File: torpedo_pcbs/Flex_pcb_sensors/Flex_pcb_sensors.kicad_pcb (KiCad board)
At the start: 2 copper layers, 38.1 x 23.8 mm, 10 parts, among them IC1 VL53L1CXV0FY_1, J1 Conn_01x04, J2 Conn_01x04, J3 mounting, U1 MS583702BA01-50

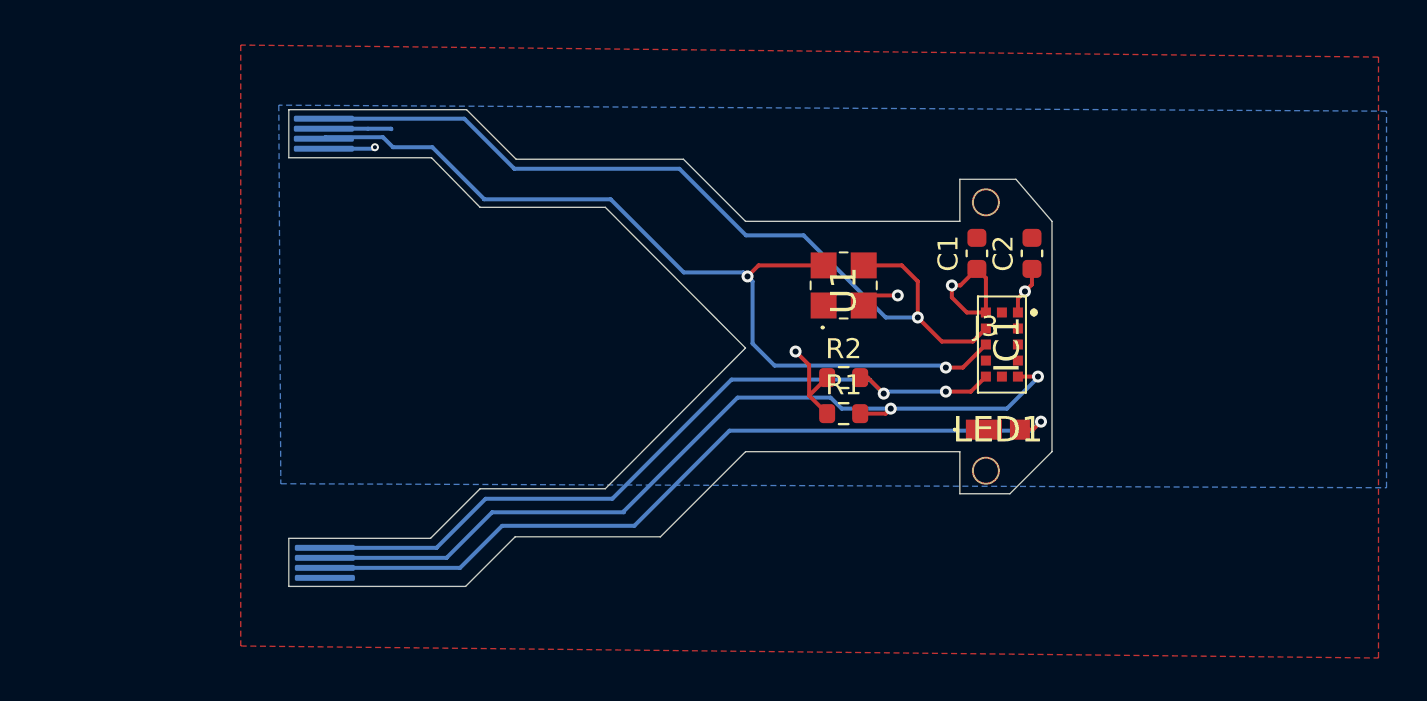
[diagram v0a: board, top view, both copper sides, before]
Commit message: everything is connected
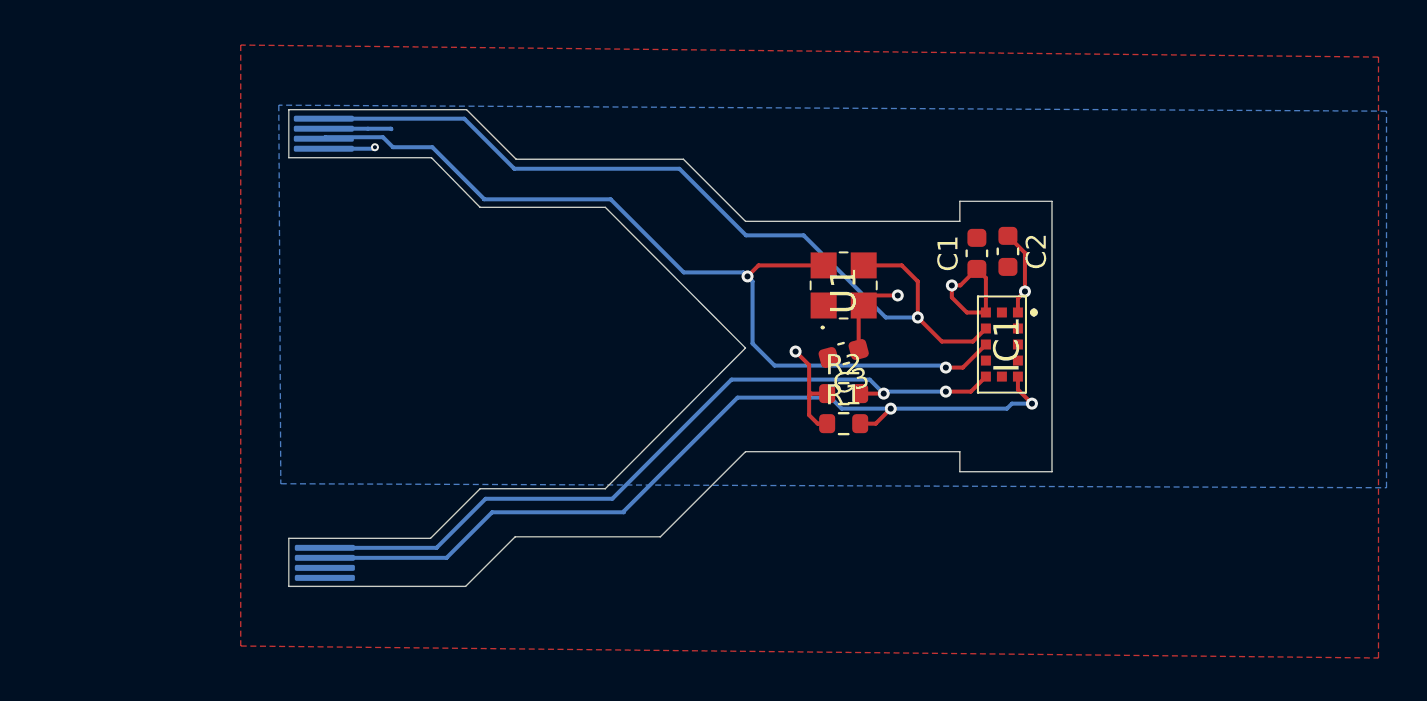
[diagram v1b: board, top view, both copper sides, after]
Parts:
- removed J3: mounting, MountingEquipment:small mounting holes
- removed LED1: 158301260A, SamacSys_Parts:158301260A
- added C3: 100nf, Capacitor_SMD:C_0603_1608Metric, F.Cu at (164.7, 80.3)
- moved C2 1.20 mm to (172.9, 75.2), turned to -90 degrees
- moved R2 0.80 mm to (164.7, 82.3)
- moved R1 0.50 mm to (164.7, 83.8)
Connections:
- J1 pad 3: Net-(J1-Pin_3) -> unconnected-(J1-Pin_3-Pad3)
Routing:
- net Net-(J1-Pin_3): track 40.0 -> 0.00 mm, vias 1 -> 0
- net +3.3V: track 19.3 -> 24.3 mm
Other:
- outline, holes or cut-outs redrawn

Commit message: June-1-2025 jlcpcb order
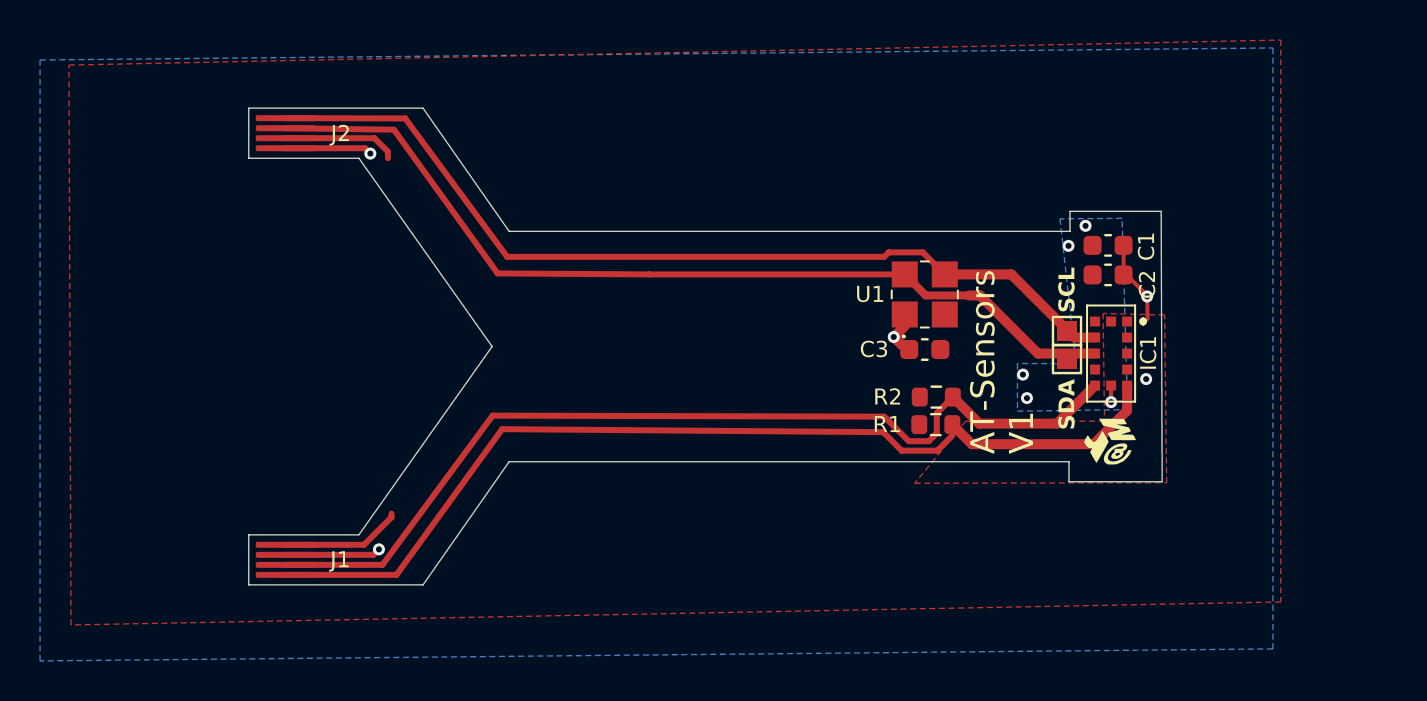
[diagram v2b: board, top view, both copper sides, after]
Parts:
- added G***: LOGO, LOGO, F.Cu at (178.0, 84.7)
- added J3: Conn_01x01, TestPoint:TestPoint_Pad_1.0x1.0mm, F.Cu at (175.8, 80.6)
- added J8: Conn_01x01, TestPoint:TestPoint_Pad_1.0x1.0mm, F.Cu at (175.8, 79.2)
- J1, J2: moved to F.Cu
- moved C1 6.56 mm to (177.9, 74.9), turned to 0 degrees
- moved IC1 5.47 mm to (178.0, 80.3)
- moved C2 5.14 mm to (177.9, 76.4), turned to 0 degrees
- moved R2 4.63 mm to (169.3, 82.5)
- moved R1 4.60 mm to (169.3, 83.8)
- moved U1 4.07 mm to (168.7, 77.3)
- moved C3 4.05 mm to (168.8, 80.1), turned to 180 degrees
- moved J1 1.96 mm to (136.8, 89.8), turned to 0 degrees
- moved J2 1.90 mm to (136.8, 68.5), turned to 0 degrees
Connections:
- J1 pad 1: /GPIO1 -> +3.3V
- J1 pad 2: /xShut -> GND
- J1 pad 3: unconnected-(J1-Pin_3-Pad3) -> /GPIO1
- J1 pad 4: unconnected-(J1-Pin_4-Pad4) -> /xShut
- J2 pad 2: +3.3V -> /SDA
- J2 pad 3: /SDA -> +3.3V
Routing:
- net GND: track 2.90 -> 16.8 mm, vias 1 -> 6
- net +3.3V: track 24.3 -> 12.7 mm
- net /GPIO1: track 38.3 -> 47.6 mm, vias 2 -> 0
- net /xShut: track 42.4 -> 49.4 mm, vias 2 -> 0
- net /SDA: track 44.2 -> 37.6 mm, vias 2 -> 0
- net /SCL: track 42.8 -> 37.3 mm, vias 1 -> 0
- added copper zone on F.Cu, net +3.3V
- added copper zone on B.Cu, net GND
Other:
- board size 38.1 x 23.8 mm -> 45.6 x 23.8 mm
- board text added: "AT-Sensors V1"
- board text added: "SCL"
- board text added: "SDA"
- board text removed: "steel stiffner"
